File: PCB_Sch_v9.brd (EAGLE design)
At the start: 38.3 x 38.1 mm, 59 parts, among them IC1 CP2104, M1 C0720B001F, Q1 MMBT2222LT1G, Q2 mmbt2222, Q3 DMG3415U, Q4 mmbt2222, U1 ESP32-WROOM-32D, U2 UG-2828GDEDF11, U3 MCP73831T-2ACI/OT, U4 AP2112-3.3, U5 FAN5331SX, X1 JSTPH, X4 20329

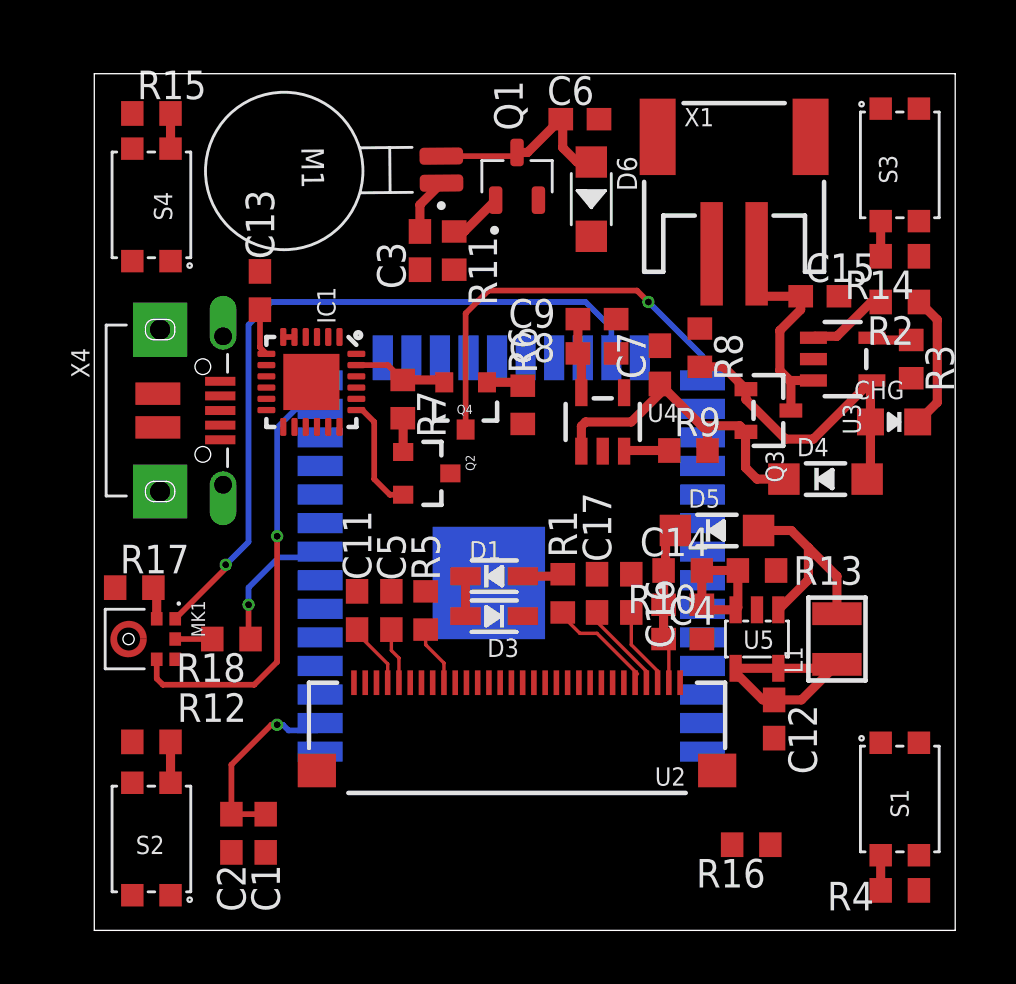
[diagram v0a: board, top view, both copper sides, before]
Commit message: Final design
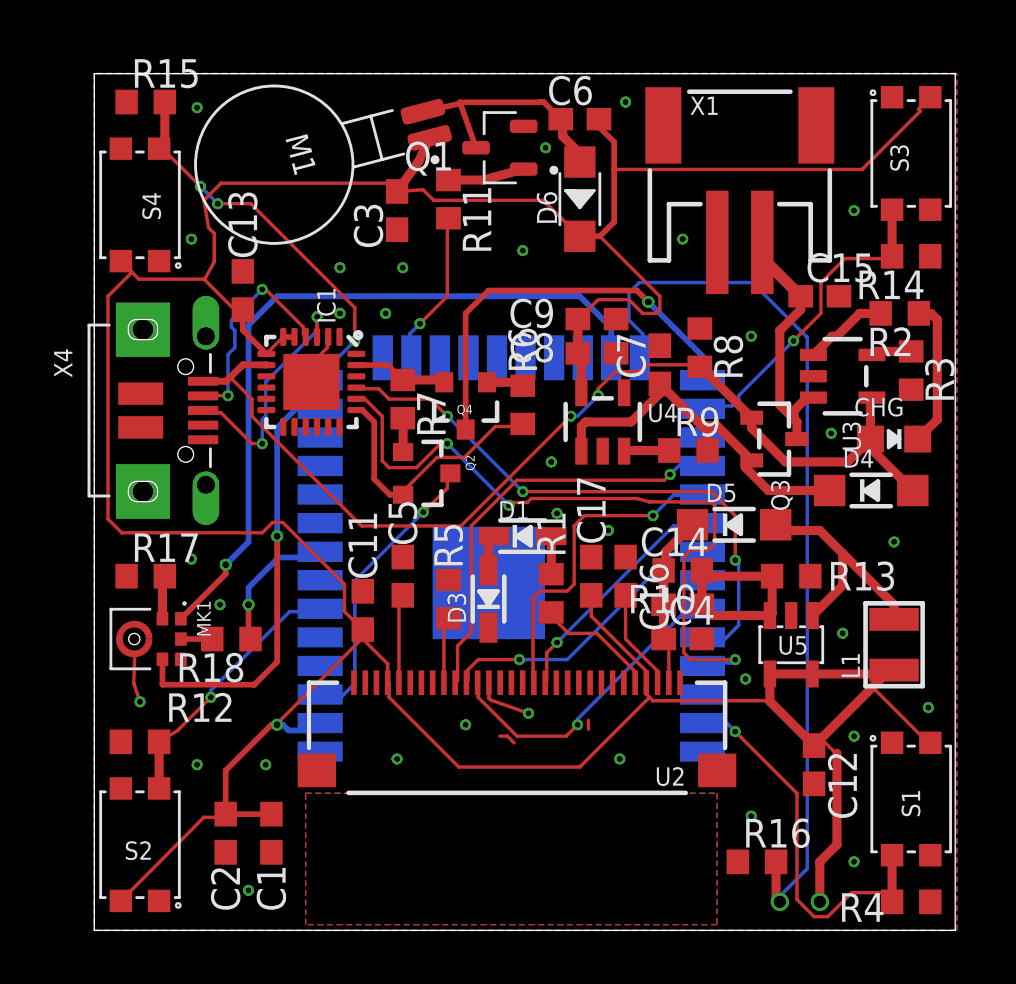
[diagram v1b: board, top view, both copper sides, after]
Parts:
- moved C12 2.70 mm to (32.0, 7.37)
- moved L1 2.55 mm to (35.6, 12.7)
- moved R11 2.30 mm to (15.7, 32.5)
- moved D1 2.18 mm to (19.1, 17.5)
- moved D4 2.09 mm to (34.5, 19.6)
- moved C3 2.05 mm to (13.5, 32.0)
- moved C5 1.61 mm to (13.7, 15.7)
- moved U5 1.55 mm to (31.0, 12.7)
- moved R13 1.55 mm to (31.0, 15.7)
- moved Q1 1.48 mm to (18.0, 34.8), turned to 180 degrees
- moved Q3 1.30 mm to (30.2, 21.8)
- moved R5 1.14 mm to (15.7, 14.7)
- moved M1 0.92 mm to (9.91, 34.5), turned to 104.7 degrees
- moved D5 0.80 mm to (28.4, 18.0)
- moved R16 0.80 mm to (29.5, 3.05), turned to 0 degrees
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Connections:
- removed net VBUS1: IC1.8, X4.VBUS
- net BTN_WRIST: now also R16.2
- net VBUS: now also IC1.8, X4.VBUS
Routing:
- net 3.3V: track 34.2 -> 172.1 mm, vias 1 -> 2
- net BTN_WRIST: track 0.00 -> 39.8 mm, vias 0 -> 1
- net TXD0: track 0.00 -> 31.7 mm, vias 0 -> 3
- net VBUS: track 14.8 -> 45.3 mm, vias 0 -> 2
- net RXD0: track 0.00 -> 26.0 mm, vias 0 -> 3
- net OLED_RES: track 0.00 -> 18.7 mm, vias 0 -> 1
- net BTN_UL: track 1.56 -> 17.8 mm, vias 0 -> 3
- net BTN_LR: track 1.56 -> 17.5 mm, vias 0 -> 1
- net OLED_SCK: track 0.00 -> 14.7 mm, vias 0 -> 1
- net OLED_CS: track 0.00 -> 13.9 mm, vias 0 -> 1
- net OLED_DC: track 0.00 -> 13.2 mm, vias 0 -> 1
- net RESET: track 0.00 -> 13.0 mm, vias 0 -> 1
- net BTN_UR: track 1.56 -> 14.2 mm, vias 0 -> 1
- net N$1: track 0.00 -> 10.8 mm, vias 0 -> 2
- net OLED_MOSI: track 0.00 -> 10.7 mm, vias 0 -> 1
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- added copper zone on layer 1, net CUT
- added copper zone on layer 16, net CUT
- added copper zone on layer 1, net GND
- added copper zone on layer 16, net GND
